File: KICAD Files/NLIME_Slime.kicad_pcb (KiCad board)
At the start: 2 copper layers, 32.5 x 34.5 mm, 28 parts, among them SW2 SWO, SW3 SW_Push, U2 QMC6309, U3 ICM-45686, X1 32.768MHz

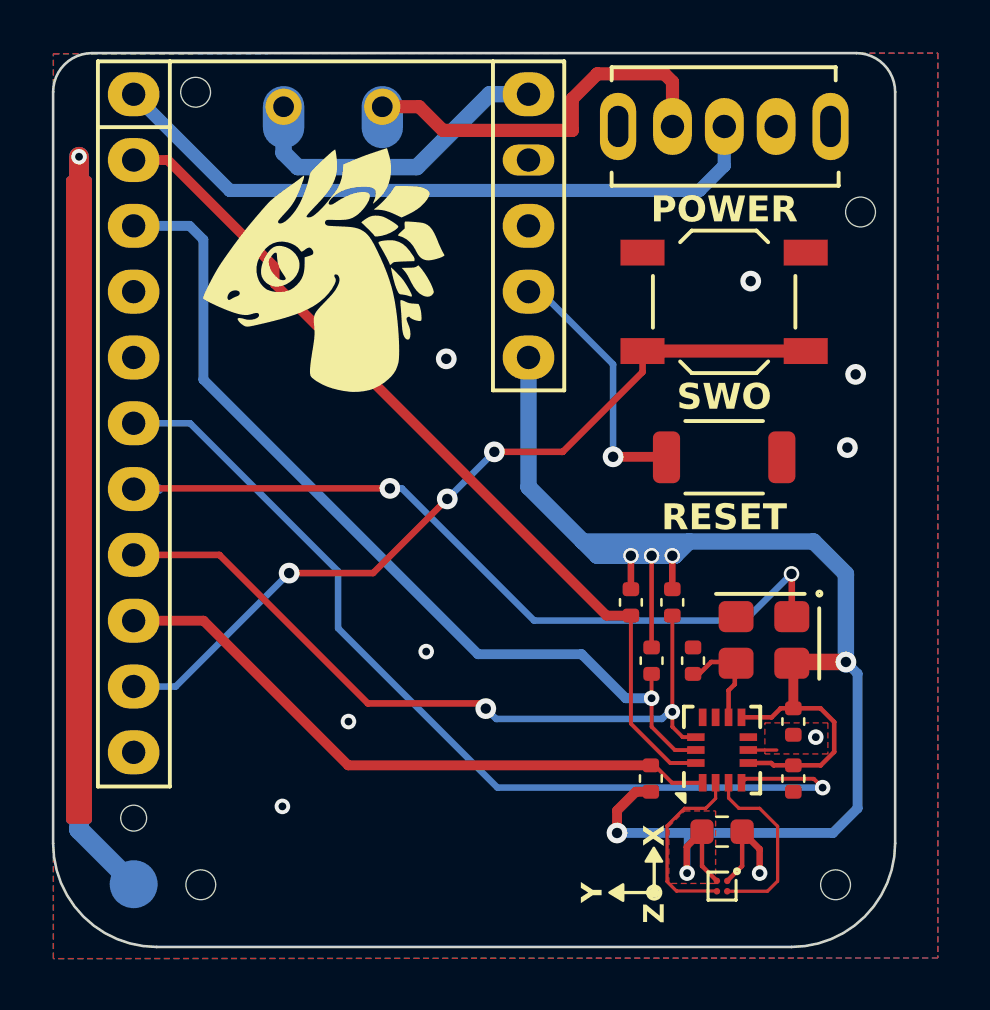
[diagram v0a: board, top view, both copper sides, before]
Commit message: Add files via upload
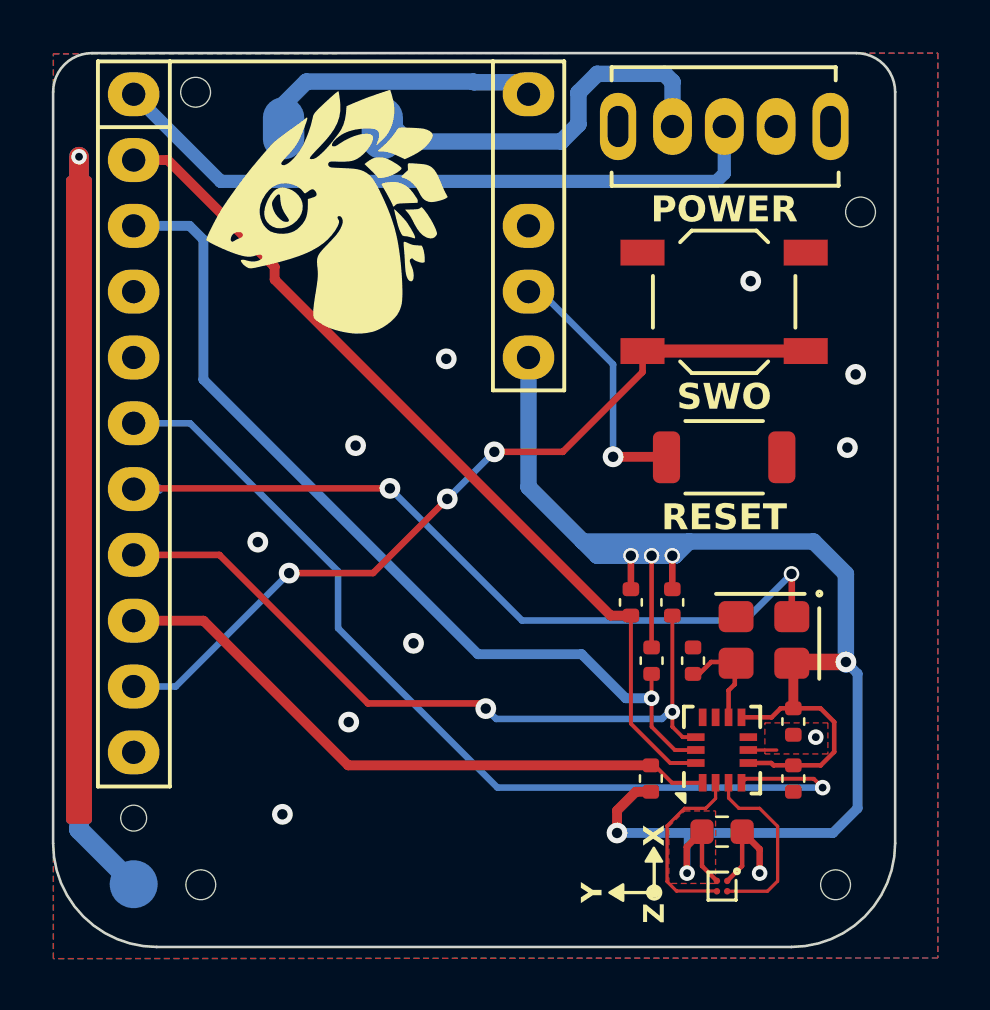
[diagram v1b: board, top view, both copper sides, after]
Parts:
- moved G*** 2.25 mm to (21.6, 21.2)
- moved BT1 0.43 mm to (21.8, 17.5)
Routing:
- net +BATT: track 12.6 -> 10.1 mm
- net GND: vias 9 -> 11
